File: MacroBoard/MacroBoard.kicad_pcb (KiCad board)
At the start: 2 copper layers, 103.3 x 105.9 mm, 116 parts, among them J1 TYPE-C-31-M12_13, SW1 SW_Push, SW2 RotaryEncoder_Switch, SW3 RotaryEncoder_Switch, U1 AT90USB1286-AU, U2 TPD4E05U06DQAR, Y1 Crystal_GND24_Small

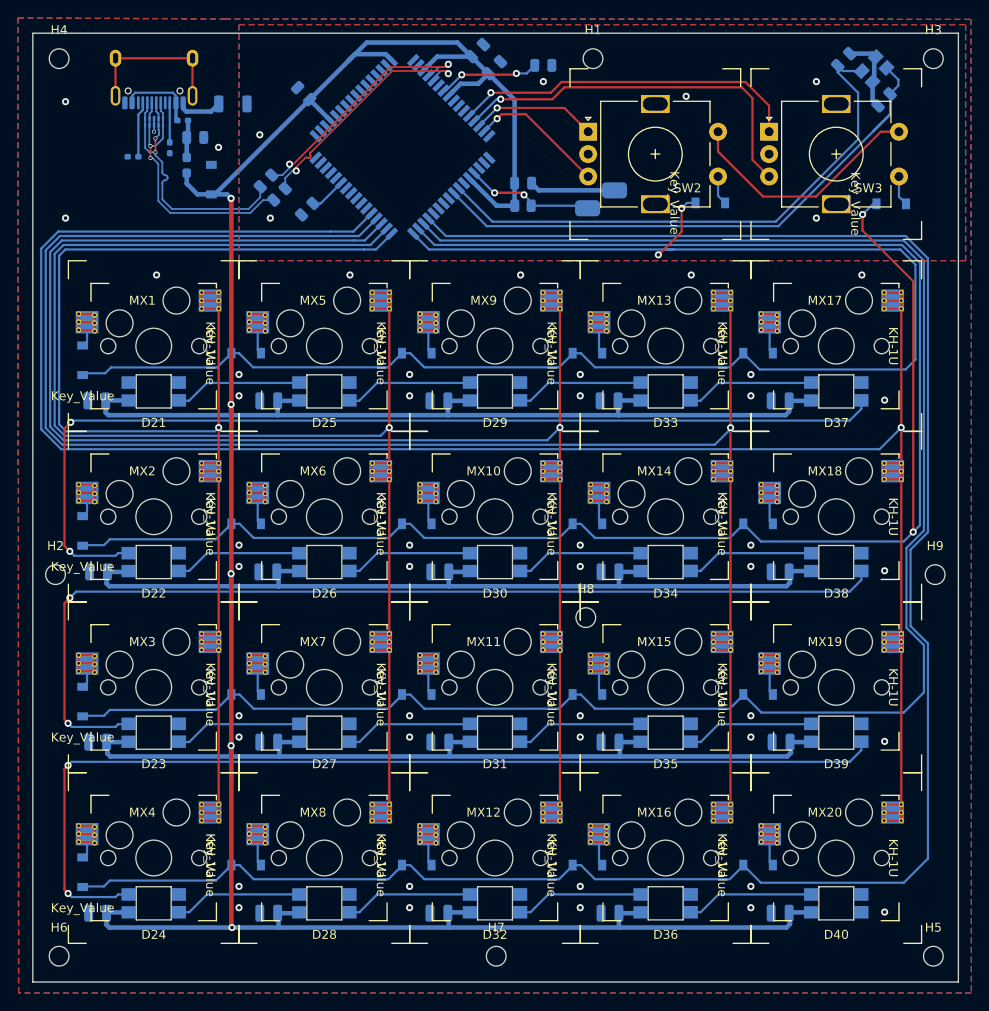
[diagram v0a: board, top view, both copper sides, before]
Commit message: minor changes
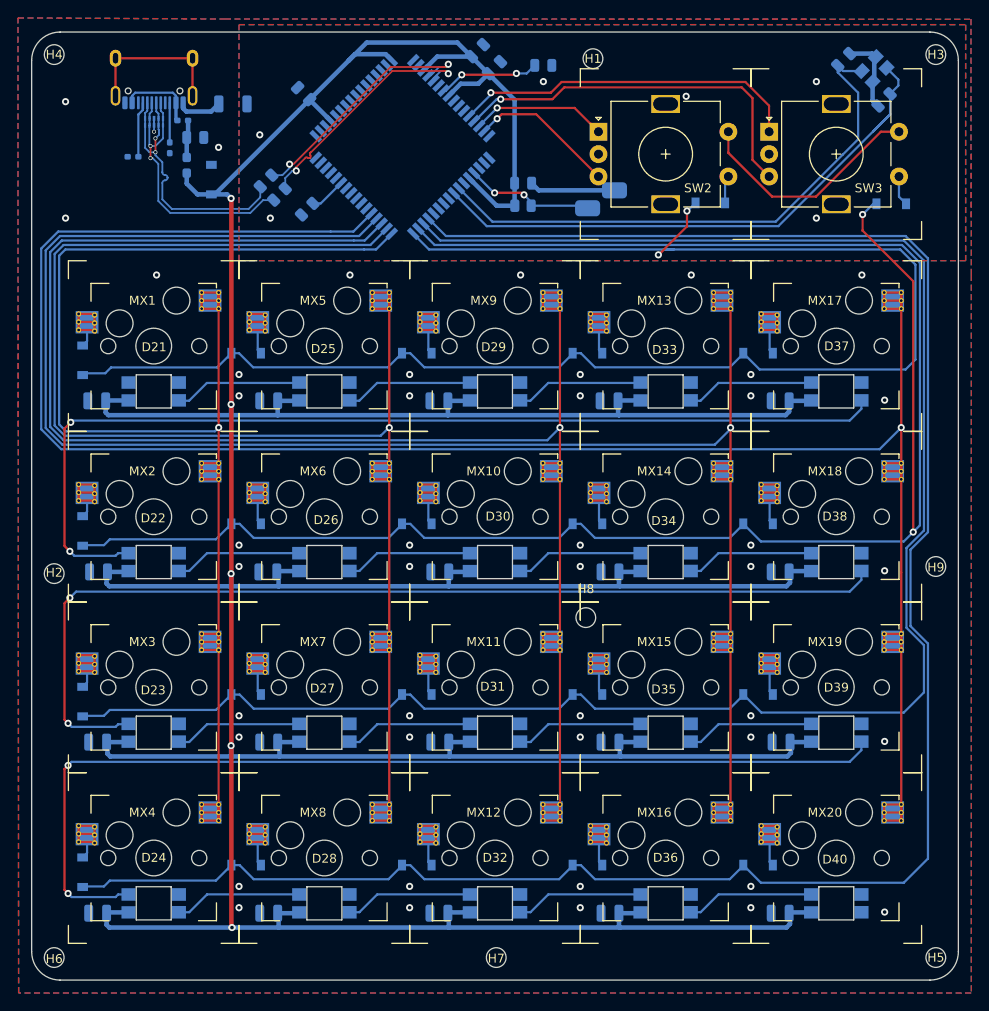
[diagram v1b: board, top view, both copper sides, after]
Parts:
- moved SW2 1.15 mm to (138.1, 43.7)
- moved H9 0.91 mm to (168.3, 89.7)
- moved H4 0.71 mm to (69.8, 32.5)
- moved H6 0.57 mm to (69.8, 133.3)
- moved H3 0.53 mm to (168.3, 32.5)
- moved H5 0.31 mm to (168.3, 133.3)
- moved H2 0.19 mm to (69.8, 90.5)
- moved H7 0.15 mm to (119.2, 133.3)
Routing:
- net /ROT_1B: track 15.3 -> 16.4 mm
- net /ROT_1A: track 14.1 -> 15.3 mm
- net Net-(SW2-PadS2): track 27.5 -> 26.4 mm
- net ROW0: track 177.2 -> 176.7 mm
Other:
- board size 103.3 x 105.9 mm -> 103.5 x 105.8 mm
